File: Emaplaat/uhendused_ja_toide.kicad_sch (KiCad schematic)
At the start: 25 parts, among them IC4 FT232RNL-TUBE, IC5 TPS54429PWPR, J1 USB-A-S-VT, J5 USB4216-03-A, J6 USB-A-S-VT, J8 Barrel_Jack

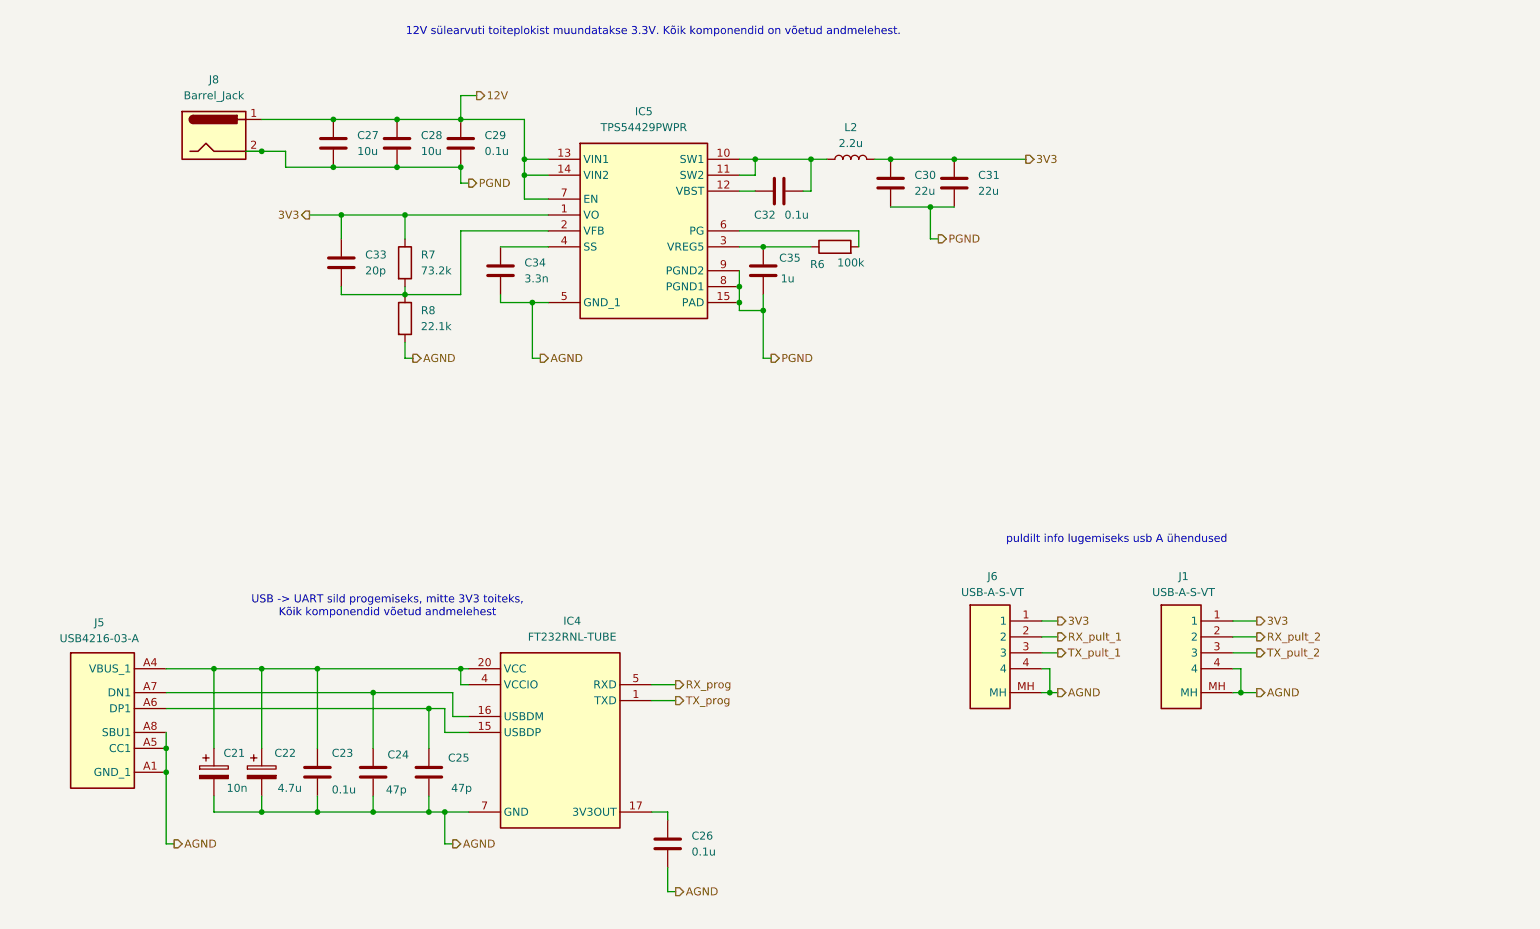
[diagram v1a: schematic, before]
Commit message: enamvahem valmis
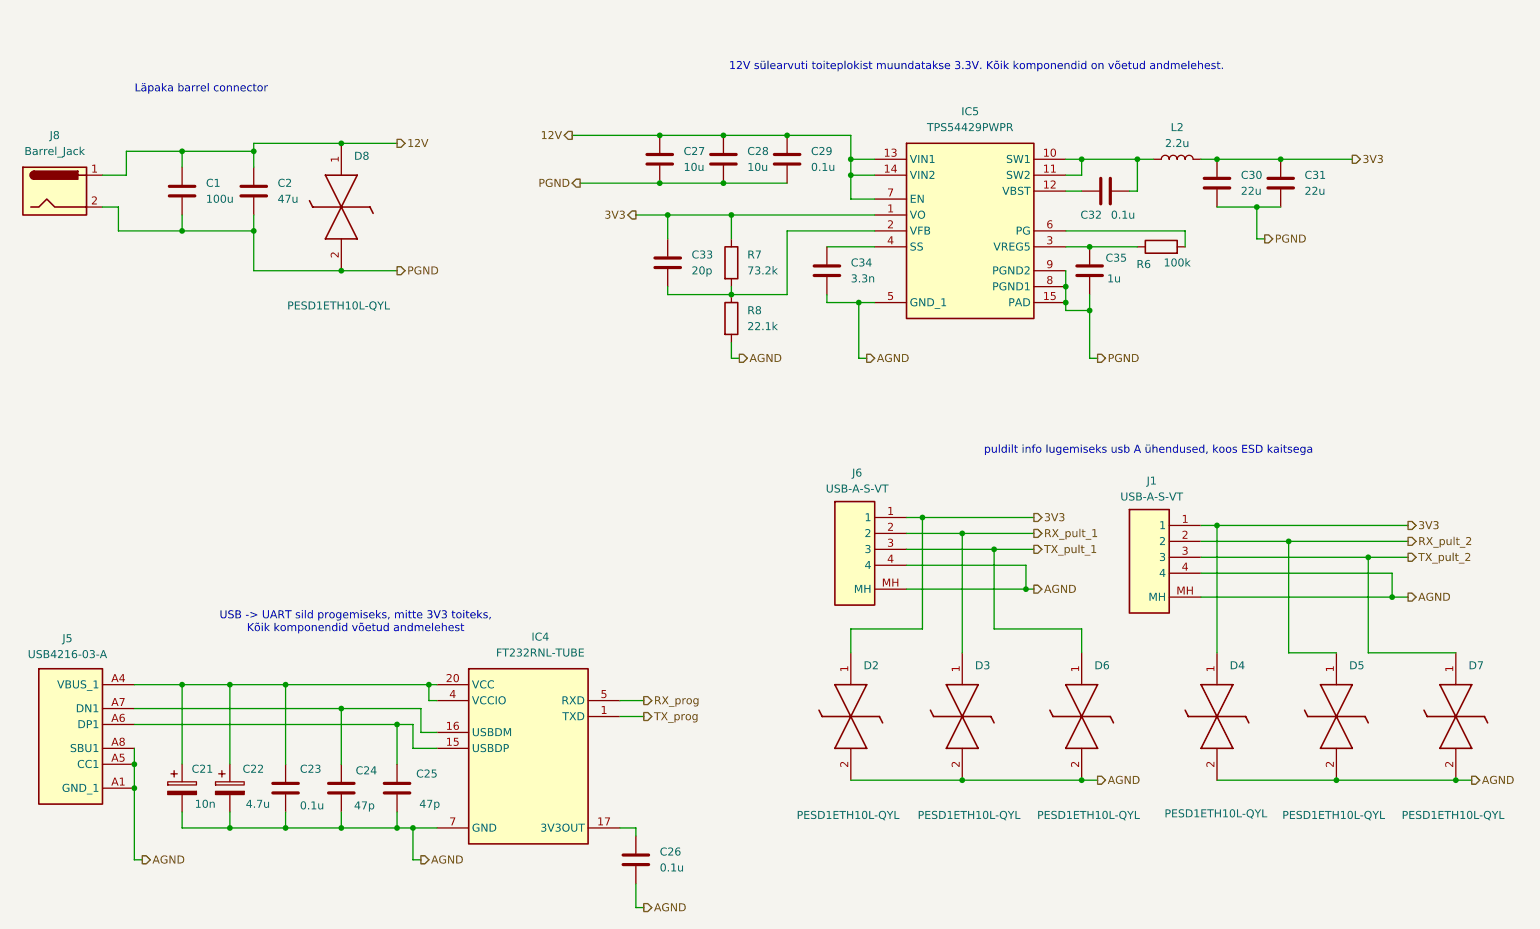
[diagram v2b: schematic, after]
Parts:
- added C1: 100u, symbol Device:C
- added C2: 47u, symbol Device:C
- added D2, D3, D4, D5, D6, D7, D8: PESD1ETH10L-QYL, PESD1ETH10LQYL, symbol PESD1ETH10L-QYL:PESD1ETH10L-QYL
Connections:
- net 12V: now also C1.1, C2.1, D8.1 (K1)
- net 3V3: now also D2.1 (K1), D4.1 (K1)
- net AGND: now also D2.2 (K2), D3.2 (K2), D4.2 (K2), D5.2 (K2), D6.2 (K2), D7.2 (K2)
- net PGND: now also C1.2, C2.2, D8.2 (K2)
- net RX_pult_1: now also D3.1 (K1)
- net RX_pult_2: now also D5.1 (K1)
- net TX_pult_1: now also D6.1 (K1)
- net TX_pult_2: now also D7.1 (K1)
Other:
- note added: "Läpaka barrel connector"
- note added: "puldilt info lugemiseks usb A ühendused, koos ESD kaitsega"
- note removed: "puldilt info lugemiseks usb A ühendused"
- moved on the sheet: C21, C22, C23, C24, C25, C26, C27, C28, C29, C30, C31, C32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

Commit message: git stuff
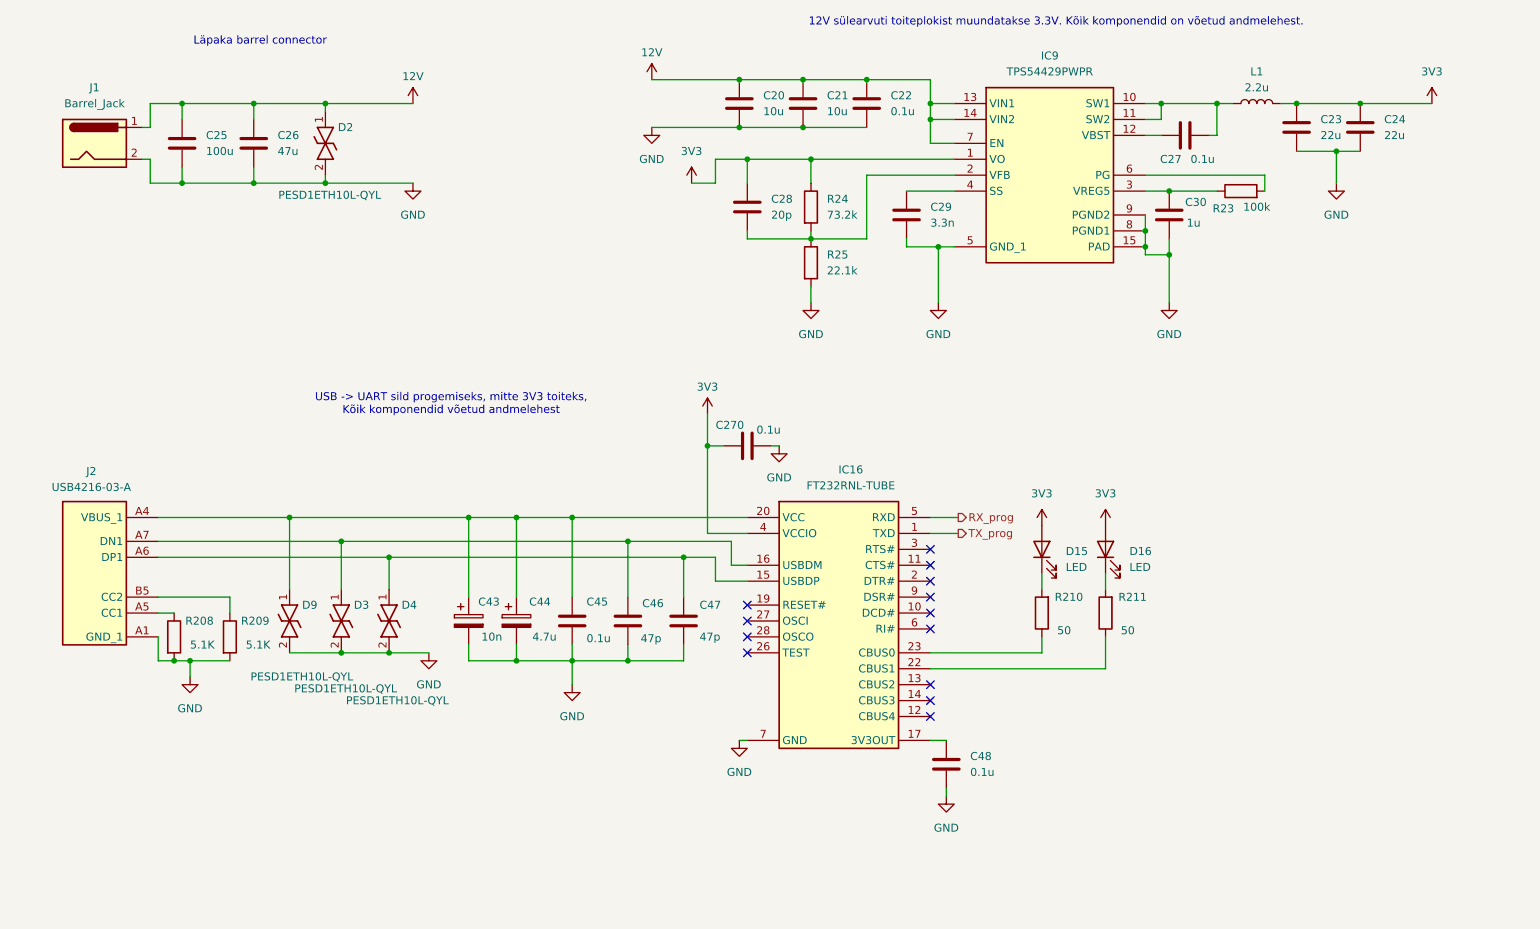
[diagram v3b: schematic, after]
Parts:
- removed D5, D6, D7, D8: PESD1ETH10L-QYL, PESD1ETH10LQYL, symbol PESD1ETH10L-QYL:PESD1ETH10L-QYL
- removed J1, J6: USB-A-S-VT, USBASVT, symbol USB-A-S-VT:USB-A-S-VT
- added C270: 0.1u, symbol Device:C
- added D15, D16: LED, LED_SMD:LED_0603_1608Metric, symbol Device:LED
- added D9: PESD1ETH10L-QYL, PESD1ETH10LQYL, symbol PESD1ETH10L-QYL:PESD1ETH10L-QYL
- added R208, R209: 5.1K, symbol Device:R
- added R210, R211: 50, Resistor_SMD:R_0603_1608Metric, symbol Device:R
- renumbered C27 to C20, C28 to C21, C29 to C22, C30 to C23, C31 to C24, C1 to C25, C2 to C26, C32 to C27, C33 to C28, C34 to C29, C35 to C30, C21 to C43, C22 to C44, C23 to C45, C24 to C46, C25 to C47, C26 to C48, IC4 to IC16, IC5 to IC9, J8 to J1, J5 to J2, L2 to L1, R6 to R23, R7 to R24, R8 to R25
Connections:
- net PGND is gone; now on net AGND: C20.2, C21.2, C22.2, C23.2, C24.2, C25.2, C26.2, C30.2, IC9.15 (PAD), IC9.8 (PGND1), IC9.9 (PGND2), J1.2
- net RX_pult_1 is gone; now on an unnamed net: D3.1 (K1)
- net 12V: now also D2.1 (K1)
- net 3V3: now also IC16.4 (VCCIO), C270.1, D15.2 (A), D16.2 (A); no longer D2.1 (K1), D4.1 (K1)
- net AGND: now also C270.2, D9.2 (K2), R208.2, R209.2; no longer IC16.26 (TEST), IC16.28 (OSCO), J2.A5 (CC1), J2.A8 (SBU1), J2.B5 (CC2), J2.B8 (SBU2)
- net at C43.1, C44.1, C45.1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: now also D9.1 (K1); no longer IC16.4 (VCCIO)
- net at C47.1, IC16.15 (USBDP), J2.A6 (DP1)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: now also D4.1 (K1)
- net at IC16.24 (NC_2), IC16.8 (NC_1): no longer IC16.19 (RESET#), IC16.27 (OSCI)
- new net: J2.B5 (CC2), R209.1
- new net: J2.A5 (CC1), R208.1
- new net: IC16.23 (CBUS0), R210.1
- new net: D15.1 (K), R210.2
- new net: IC16.22 (CBUS1), R211.1
- new net: J2.A8 (SBU1), J2.B8 (SBU2)
- new net: D16.1 (K), R211.2
- now unconnected: IC16.10 (DCD#), IC16.11 (CTS#), IC16.12 (CBUS4), IC16.13 (CBUS2), IC16.14 (CBUS3), IC16.2 (DTR#), IC16.3 (RTS#), IC16.6 (RI#), IC16.9 (DSR#)
- no-connect marks 0 -> 13
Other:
- note removed: "puldilt info lugemiseks usb A ühendused, koos ESD kaitsega"
- moved on the sheet: C20, C21, C22, C23, C24, C25, C26, C27, C28, C29, C30, C43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
